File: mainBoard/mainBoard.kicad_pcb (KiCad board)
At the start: 4 copper layers, 50 x 60 mm, 61 parts, among them J1 Conn_01x04, J10 Conn_02x07_Odd_Even, J2 Conn_01x04, J6 Conn_01x07, J7 Conn_01x07, J8 Conn_01x02, J9 Conn_01x08, M1 Conn_01x01, M2 Conn_01x01, U1 MAX15062A, U2 STM32H503CBT6, U3 DRV8251ADDAR

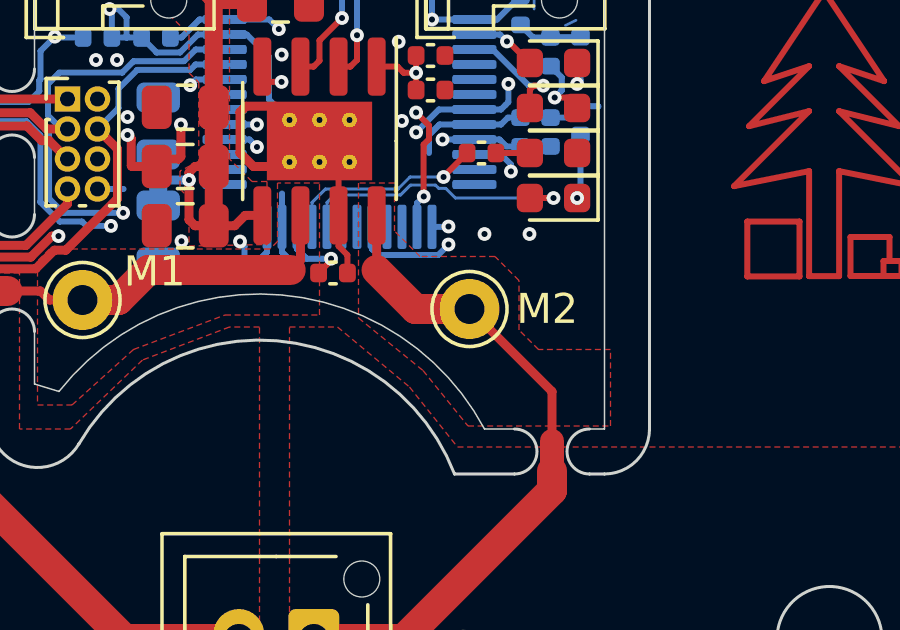
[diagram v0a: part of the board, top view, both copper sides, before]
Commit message: GNDDETECT
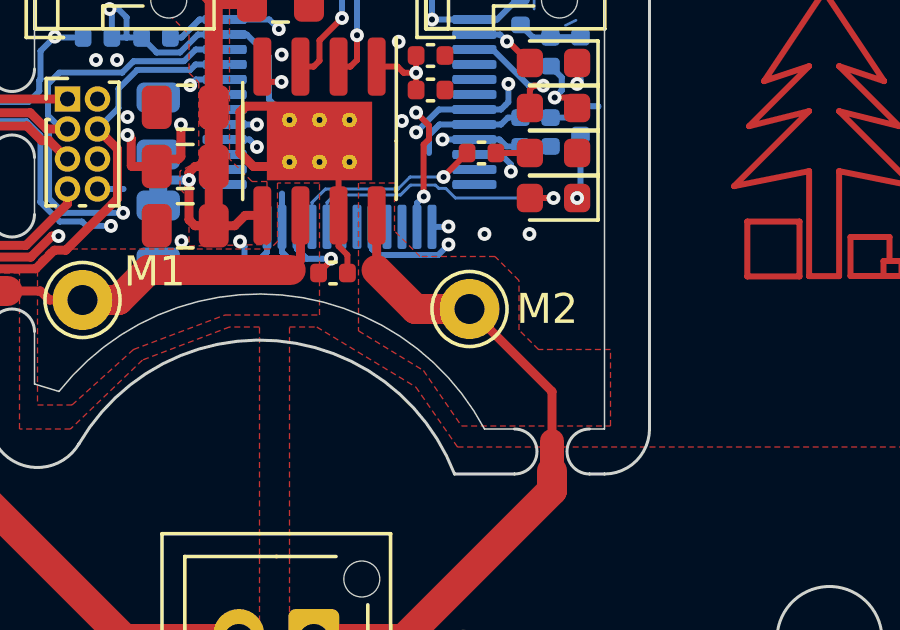
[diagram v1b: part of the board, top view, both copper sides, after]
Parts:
- removed C34: 2u2, Capacitor_SMD:C_0805_2012Metric
- added C21: 2u2, Capacitor_SMD:C_0805_2012Metric, B.Cu at (152.7, 88.5)
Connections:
- J10 pad 11: unconnected-(J10-Pin_11-Pad11) -> GND

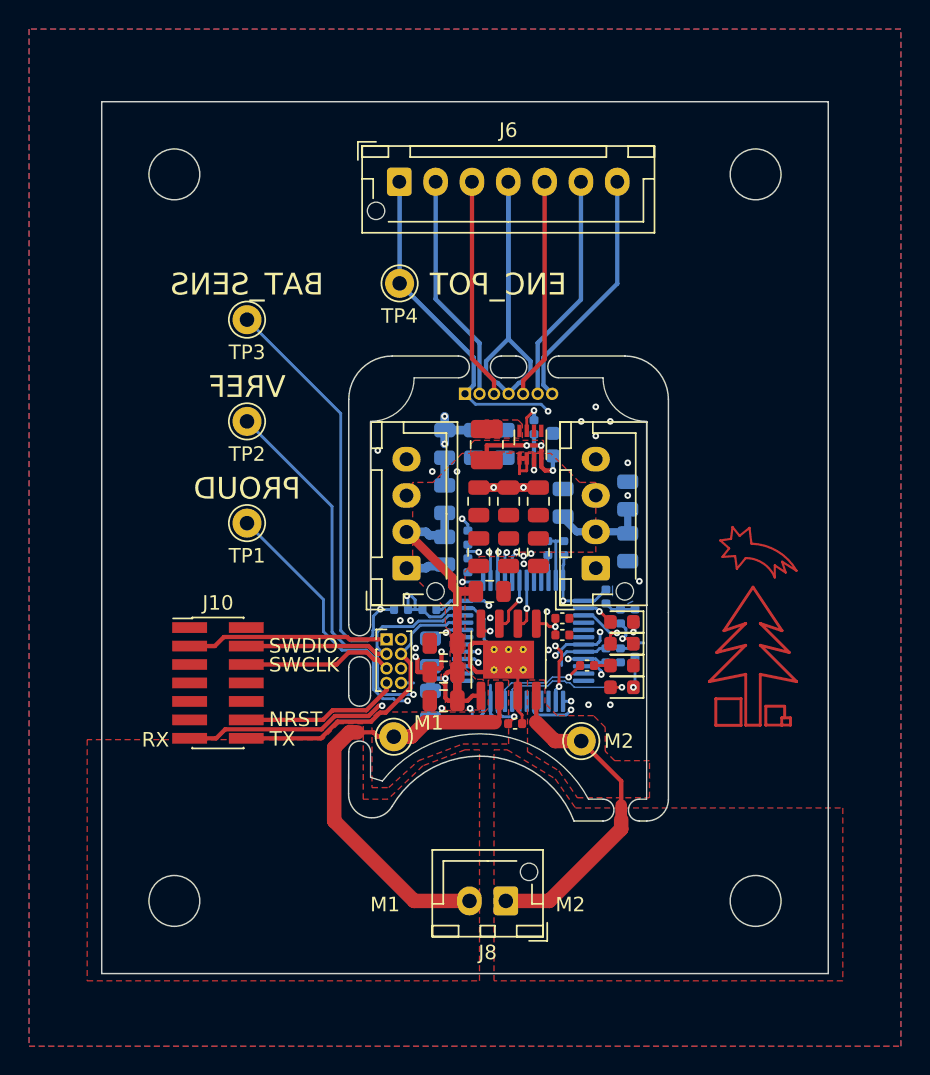
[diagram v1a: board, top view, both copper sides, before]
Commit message: 16x20
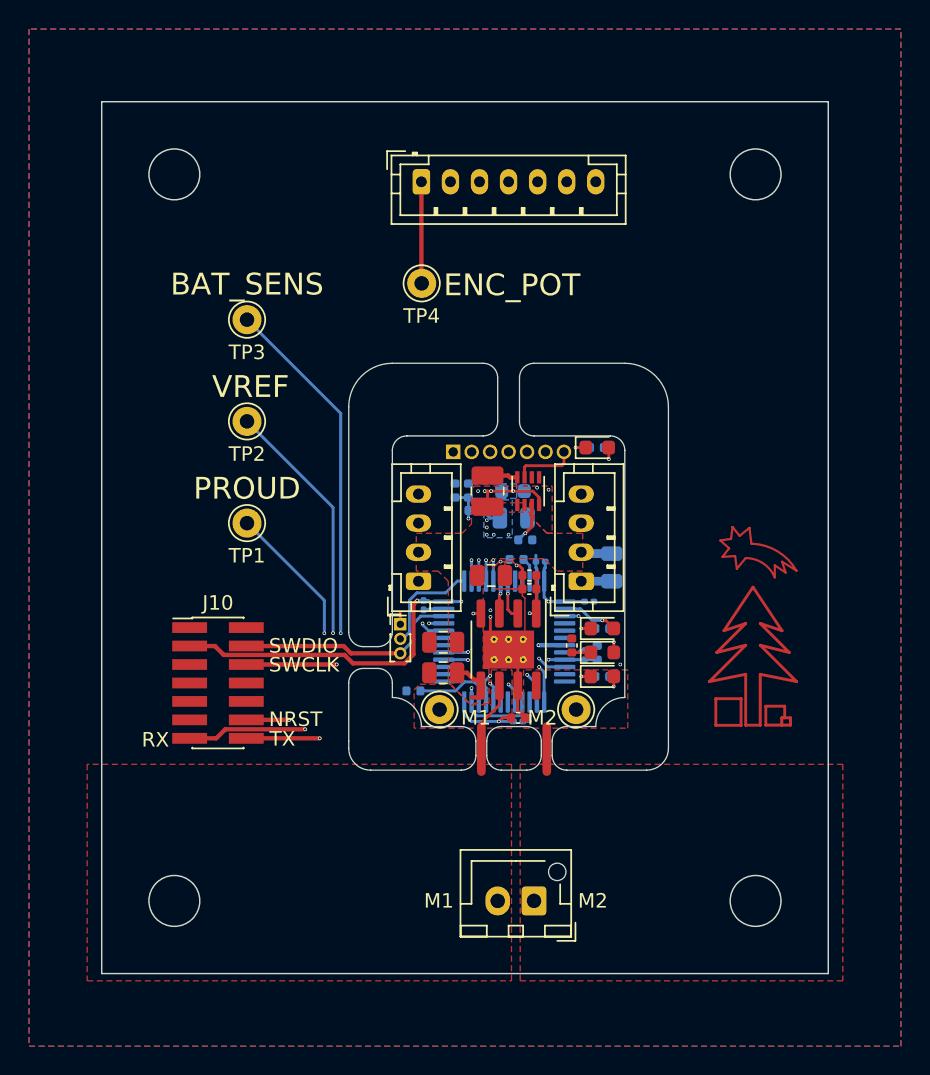
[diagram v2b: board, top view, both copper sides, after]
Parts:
- removed C19, C20, C21, C22, C23, C24, C25, C26, C27, C28, C29, C30, C31, C32, C33: 2u2, Capacitor_SMD:C_0805_2012Metric
- removed J9: Conn_01x08, Connector_PinHeader_1.00mm:PinHeader_2x04_P1.00mm_Vertical
- added J3: Conn_01x03, Connector_PinHeader_1.00mm:PinHeader_1x03_P1.00mm_Vertical, F.Cu at (145.6, 101.0)
- C10, C6, C7, C8, C9: footprint Capacitor_SMD:C_0402_1005Metric -> Capacitor_SMD:C_0201_0603Metric
- C11, R6: moved to B.Cu
- C14: value 2u2 -> 10u; moved to B.Cu
- C16, C17, C18: value 2u2 -> 10u
- C5, R5: moved to F.Cu
- J1, J2: footprint Connector_JST:JST_XH_B4B-XH-AM_1x04_P2.50mm_Vertical -> Connector_JST:JST_PH_B4B-PH-K_1x04_P2.00mm_Vertical
- J6: footprint Connector_JST:JST_XH_B7B-XH-AM_1x07_P2.50mm_Vertical -> Connector_JST:JST_PH_B7B-PH-K_1x07_P2.00mm_Vertical
- J7: footprint Connector_PinHeader_1.00mm:PinHeader_1x07_P1.00mm_Vertical -> Connector_PinHeader_1.27mm:PinHeader_1x07_P1.27mm_Vertical
- moved D4 15.1 mm to (159.1, 88.8), turned to 0 degrees
- moved R6 15.0 mm to (159.1, 88.8)
- moved C17 13.5 mm to (148.5, 104.3), turned to 180 degrees
- moved J1 12.2 mm to (146.8, 98.0)
- moved J2 12.1 mm to (158.0, 98.0)
- moved C8 11.7 mm to (155.2, 96.7), turned to 180 degrees
- moved C6 11.0 mm to (158.6, 99.4), turned to 0 degrees
- moved C16 10.7 mm to (148.5, 102.2), turned to 180 degrees
- moved C7 10.5 mm to (153.7, 107.7), turned to 0 degrees
- moved C9 10.4 mm to (147.2, 99.7), turned to -90 degrees
- moved C14 10.2 mm to (160.1, 97.0), turned to -90 degrees
- moved C1 9.41 mm to (150.2, 91.8), turned to 90 degrees
- moved C2 8.10 mm to (153.3, 93.7), turned to 0 degrees
- moved C3 7.77 mm to (154.2, 95.2), turned to 0 degrees
- moved C11 7.35 mm to (146.4, 105.5), turned to 180 degrees
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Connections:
- D4 pad 1: GND -> Net-(D4-K)
- D4 pad 2: Net-(D4-A) -> /CPU/LED.Y
- R6 pad 1: /CPU/LED.Y -> Net-(D4-K)
- R6 pad 2: Net-(D4-A) -> GND
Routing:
- net VCC: track 51.5 -> 8.02 mm, vias 4 -> 5
- net Net-(J8-Pin_2): track 30.6 -> 6.43 mm
- net /CPU/LED.Y: track 6.67 -> 26.9 mm, vias 1 -> 3
- net GND: track 82.6 -> 62.6 mm, vias 23 -> 5
- net Net-(J8-Pin_1): track 22.6 -> 3.10 mm
- net /CPU/ENC.MISO: track 45.0 -> 28.1 mm
- net VDD: track 102.2 -> 91.7 mm, vias 7 -> 10
- net /CPU/MEŘENÍ-NAPÁJENÍ: track 61.0 -> 53.4 mm, vias 5 -> 3
- net /CPU/UART.RX: track 34.3 -> 26.7 mm, vias 2 -> 1
- net /CPU/UART.TX: track 31.4 -> 23.9 mm, vias 2 -> 1
- net /CPU/SWCLK: track 22.9 -> 18.7 mm
- net Net-(C11-Pad1): track 2.66 -> 5.49 mm, vias 1 -> 0
- net /CPU/SWDIO: track 18.1 -> 15.5 mm
- net /CPU/DRV.VREF: track 44.0 -> 41.4 mm, vias 4 -> 3
- net Net-(U1-LX): track 0.00 -> 2.10 mm
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- added copper zone on B.Cu, net VCC
- added copper zone on B.Cu, net VDD
- removed copper zone on F.Cu, net Net-(U1-LX)
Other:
- outline, holes or cut-outs redrawn
- board text removed: "G"
- board text removed: "R"
- board text removed: "T"
